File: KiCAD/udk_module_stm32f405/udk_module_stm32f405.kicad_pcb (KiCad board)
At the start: 4 copper layers, 54 x 38 mm, 33 parts, among them J1 USB_C_Receptacle, J2 5V, J3 ARGB, J4 QWIIC, J5 CONN, J6 SPI, U1 AMS1117-3.3, U2 NC7SZ125M5X, U3 STM32F405RGTx, U4 USB3300-EZK, U5 TS3USB30EDGSR

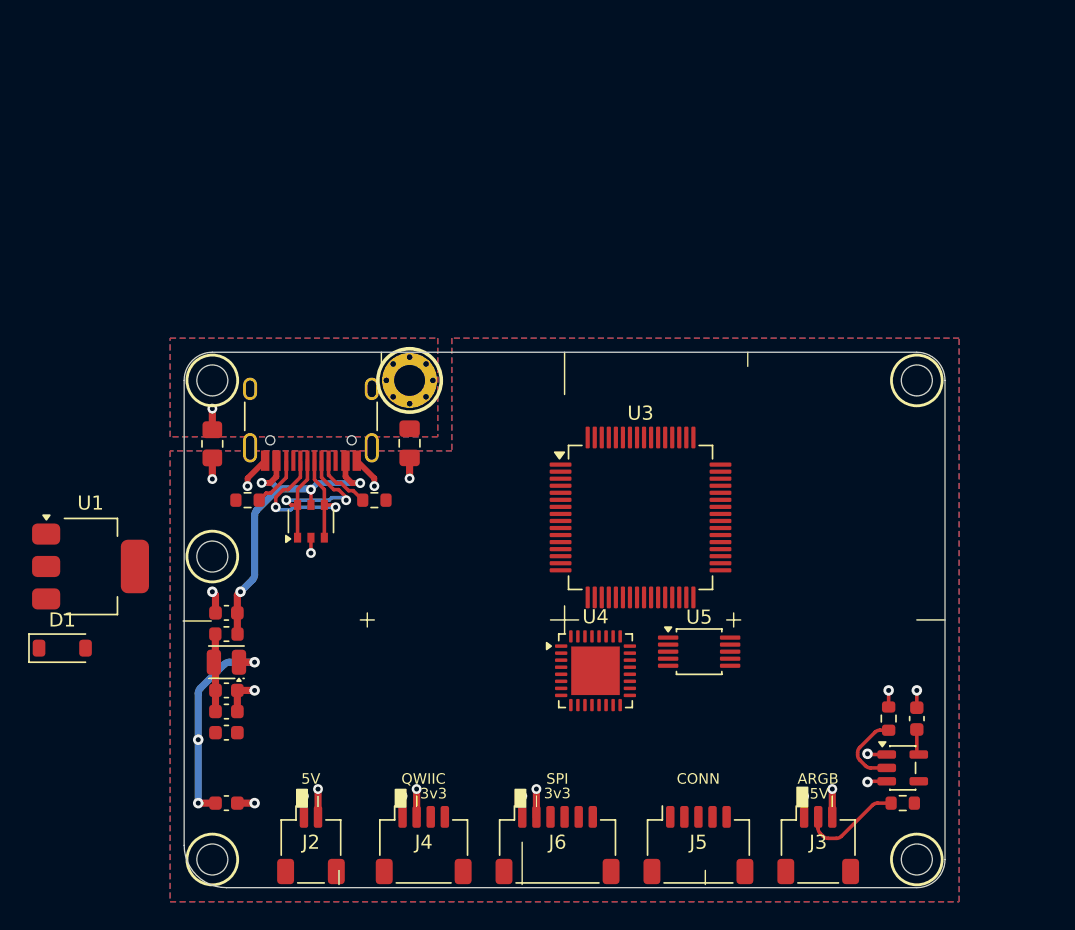
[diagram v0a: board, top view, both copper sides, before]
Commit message: wip-2025-11-27
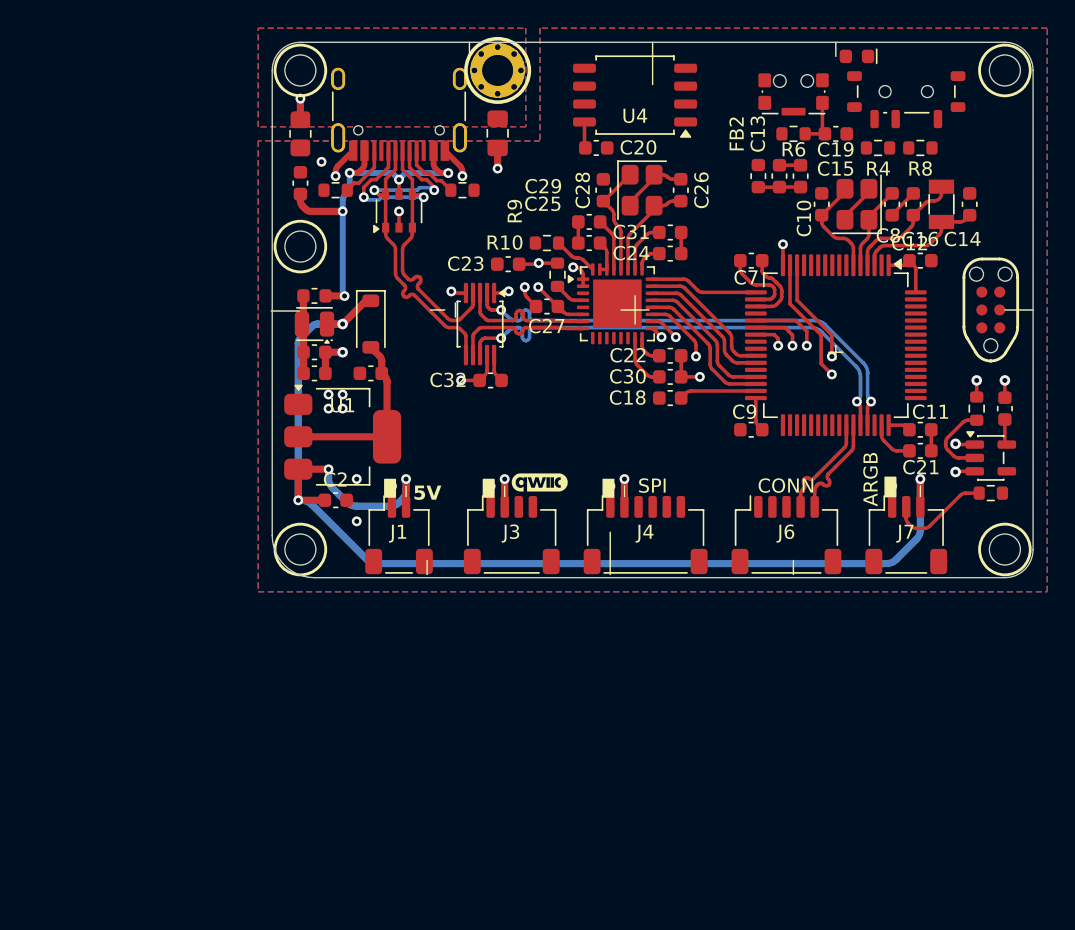
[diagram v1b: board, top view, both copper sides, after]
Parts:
- removed the U3 at (102.4, 81.7)
- added BOOT1: SW-BOOT, Button_Switch_SMD:SW_SPDT_Shouhan_MSK12C02, F.Cu at (121.2, 51.5)
- added C10: 20p, Capacitor_SMD:C_0603_1608Metric, F.Cu at (115.2, 59.5)
- added C11: 100n, Capacitor_SMD:C_0603_1608Metric, F.Cu at (122.2, 75.5)
- added C12: 100n, Capacitor_SMD:C_0603_1608Metric, F.Cu at (122.2, 63.5)
- added C13: 10n, Capacitor_SMD:C_0603_1608Metric, F.Cu at (112.2, 57.5)
- added C14: 12p, Capacitor_SMD:C_0603_1608Metric, F.Cu at (125.8, 59.5)
- added C15: 1u, Capacitor_SMD:C_0603_1608Metric, F.Cu at (113.8, 57.5)
- added C16: 12p, Capacitor_SMD:C_0603_1608Metric, F.Cu at (121.8, 59.5)
- added C18: 2u2, Capacitor_SMD:C_0603_1608Metric, F.Cu at (104.5, 73.2)
- added C19: 100n, Capacitor_SMD:C_0603_1608Metric, F.Cu at (116.2, 54.5)
- added C20: 100n, Capacitor_SMD:C_0603_1608Metric, F.Cu at (99.2, 55.5)
- added C21: 2u2, Capacitor_SMD:C_0603_1608Metric, F.Cu at (122.2, 77.0)
- added C22: 100n, Capacitor_SMD:C_0603_1608Metric, F.Cu at (104.5, 70.2)
- added C23: 1u, Capacitor_SMD:C_0603_1608Metric, F.Cu at (93.0, 63.8)
- added C24: 100n, Capacitor_SMD:C_0603_1608Metric, F.Cu at (104.5, 63.0)
- added C25: 100n, Capacitor_SMD:C_0603_1608Metric, F.Cu at (98.8, 62.2)
- added C26: 9p, Capacitor_SMD:C_0603_1608Metric, F.Cu at (105.2, 58.5)
- added C27: 100n, Capacitor_SMD:C_0603_1608Metric, F.Cu at (95.8, 66.8)
- added C28: 9p, Capacitor_SMD:C_0603_1608Metric, F.Cu at (99.8, 58.5)
- added C29: 4u7, Capacitor_SMD:C_0603_1608Metric, F.Cu at (98.8, 60.8)
- added C30: 4u7, Capacitor_SMD:C_0603_1608Metric, F.Cu at (104.5, 71.8)
- added C31: 4u7, Capacitor_SMD:C_0603_1608Metric, F.Cu at (104.5, 61.5)
- added C32: 100n, Capacitor_SMD:C_0603_1608Metric, F.Cu at (91.8, 72.0)
- added C7: 100n, Capacitor_SMD:C_0603_1608Metric, F.Cu at (110.2, 63.5)
- added C8: 20p, Capacitor_SMD:C_0603_1608Metric, F.Cu at (120.2, 59.5)
- added C9: 100n, Capacitor_SMD:C_0603_1608Metric, F.Cu at (110.2, 75.5)
- added D2: Blue, PCM_SparkFun-LED:LED_0603_1608Metric_Blue, F.Cu at (117.8, 49.0)
- added FB2: 1kΩ@100MHz, Inductor_SMD:L_0603_1608Metric, F.Cu at (110.8, 57.5)
- added G***: LOGO, PCM_SparkFun-Aesthetic:qwiic_4mm, F.Cu at (95.2, 79.2)
- added J5: TC2030_SWD, PCM_marbastlib-various:CON_TC2030_outlined, F.Cu at (127.2, 67.0)
- added R10: 12K, Resistor_SMD:R_0603_1608Metric, F.Cu at (95.8, 62.2)
- added R4: 10K, Resistor_SMD:R_0603_1608Metric, F.Cu at (119.2, 55.5)
- added R6: 10K, Resistor_SMD:R_0603_1608Metric, F.Cu at (113.2, 54.5)
- added R8: 10K, Resistor_SMD:R_0603_1608Metric, F.Cu at (122.2, 55.5)
- added R9: 820R, Resistor_SMD:R_0603_1608Metric, F.Cu at (96.5, 64.5)
- added U2: STM32F405RGTx, Package_QFP:LQFP-64_10x10mm_P0.5mm, F.Cu at (116.2, 69.5)
- added U6: USB3300-EZK, Package_DFN_QFN:QFN-32-1EP_5x5mm_P0.5mm_EP3.45x3.45mm, F.Cu at (100.8, 66.6)
- added Y1: 25MHz 20pF SMD3225-4P, Crystal:Crystal_SMD_3225-4Pin_3.2x2.5mm, F.Cu at (117.8, 59.5)
- added Y2: 32.768kHz 12.5pF SMD3215-2P, Crystal:Crystal_SMD_3215-2Pin_3.2x1.5mm, F.Cu at (123.8, 59.5)
- added Y3: 24MHz, Crystal:Crystal_SMD_3225-4Pin_3.2x2.5mm, F.Cu at (102.5, 58.5)
- added ~{RST}1: SW-RESET, Button_Switch_SMD:SW_SPST_CK_KMS2xxGP, F.Cu at (113.2, 51.5)
- C1: renamed from C4; footprint PCM_SparkFun-Capacitor:C_0603_1608Metric -> Capacitor_SMD:C_0603_1608Metric
- C17: renamed from C7; footprint PCM_SparkFun-Capacitor:C_0603_1608Metric -> Capacitor_SMD:C_0603_1608Metric
- C2: footprint PCM_SparkFun-Capacitor:C_0603_1608Metric -> Capacitor_SMD:C_0603_1608Metric
- C4: renamed from C5; footprint PCM_SparkFun-Capacitor:C_0603_1608Metric -> Capacitor_SMD:C_0603_1608Metric
- C5: renamed from C6; footprint PCM_SparkFun-Capacitor:C_0603_1608Metric -> Capacitor_SMD:C_0603_1608Metric
- C6: renamed from C3; footprint PCM_SparkFun-Capacitor:C_0603_1608Metric -> Capacitor_SMD:C_0603_1608Metric
- U4: value USB3300-EZK -> MB85RS64; footprint Package_DFN_QFN:QFN-32-1EP_5x5mm_P0.5mm_EP3.45x3.45mm -> Package_SO:SOIC-8_5.3x5.3mm_P1.27mm
- moved U4 41.0 mm to (102.0, 51.8), turned to 180 degrees
- moved D1 31.8 mm to (83.2, 68.0), turned to -90 degrees
- moved C1 30.9 mm to (78.2, 58.0), turned to 90 degrees
- moved U5 28.0 mm to (91.0, 68.0), turned to -90 degrees
- moved C6 27.5 mm to (83.2, 71.5)
- moved C4 24.8 mm to (79.2, 70.0)
- moved C5 24.8 mm to (79.2, 71.5)
- moved FB1 24.8 mm to (79.2, 66.0)
- moved PTC1 24.8 mm to (79.2, 68.0)
- moved C3 22.9 mm to (92.2, 54.5)
- moved J2 22.9 mm to (85.2, 51.6)
- moved C17 22.9 mm to (128.2, 74.0)
- moved H1 22.9 mm to (92.2, 50.0)
- moved H2 22.9 mm to (128.2, 50.0)
- moved H3 22.9 mm to (128.2, 84.0)
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- renumbered C1 to C3, J2 to J1, J1 to J2, J4 to J3, J6 to J4, J5 to J6, J3 to J7, R3 to R1, R1 to R2, R2 to R3, R4 to R5, R5 to R7, U2 to U3
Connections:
- C6 pad 1: +3.3V -> +3V3
- D1 pad 2: +3.3V -> +3V3
- J3 pad 2: +3.3V -> +3V3
- J4 pad 2: +3.3V -> +3V3
- J4 pad 4: PICO -> MISO
- J4 pad 5: POCI -> MOSI
- J4 pad 6: SS -> SS/MATRIX-CS
- J6 pad 1: CON1 -> ADC1/WKUP/CON1
- J6 pad 2: CON2 -> ADC2/CON2
- J6 pad 3: CON3 -> RGB-EN/ADC3
- R5 pad 1: unconnected-(R4-Pad1) -> RGB
- U1 pad 2: +3.3V -> +3V3
- U4 pad 1: unconnected-(U4-GND-Pad1) -> EEPROM-CS
- U4 pad 2: unconnected-(U4-GND-Pad2) -> MISO
- U4 pad 3: unconnected-(U4-CPEN-Pad3) -> GND
- U4 pad 4: unconnected-(U4-VBUS-Pad4) -> GND
- U4 pad 5: unconnected-(U4-ID-Pad5) -> MOSI
- U4 pad 6: unconnected-(U4-VDD3.3-Pad6) -> SCK
- U4 pad 7: unconnected-(U4-DP-Pad7) -> GND
- U4 pad 8: unconnected-(U4-DM-Pad8) -> +3V3
- U5 pad 1: unconnected-(U5-S-Pad1) -> USB_SELECT
- U5 pad 10: unconnected-(U5-VCC-Pad10) -> +3V3
- U5 pad 2: unconnected-(U5-D1+-Pad2) -> USB-D1+
- U5 pad 3: unconnected-(U5-D2+-Pad3) -> USB-D2+
- U5 pad 4: unconnected-(U5-D+-Pad4) -> D+
- U5 pad 5: unconnected-(U5-GND-Pad5) -> GND
- U5 pad 6: unconnected-(U5-D--Pad6) -> D-
- U5 pad 7: unconnected-(U5-D2--Pad7) -> USB-D2-
- U5 pad 8: unconnected-(U5-D1--Pad8) -> USB-D1-
- U5 pad 9: unconnected-(U5-~{OE}-Pad9) -> GND
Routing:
- net +5V: track 20.9 -> 92.6 mm, vias 5 -> 6
- net +3V3: track 0.00 -> 45.0 mm, vias 0 -> 3
- net USB-D1+: track 0.00 -> 35.0 mm, vias 0 -> 2
- net USB-D1-: track 0.00 -> 34.8 mm, vias 0 -> 2
- net GND: track 24.2 -> 51.8 mm, vias 15 -> 24
- net D-: track 14.8 -> 27.3 mm
- net D+: track 15.2 -> 27.3 mm
- net DATA3: track 0.00 -> 10.4 mm
- net DATA4: track 0.00 -> 10.4 mm
- net USB-D2-: track 0.00 -> 9.96 mm
- net USB-D2+: track 0.00 -> 9.96 mm
- net DATA1: track 0.00 -> 9.93 mm
- net DATA2: track 0.00 -> 9.93 mm
- net OSC32-IN: track 0.00 -> 9.05 mm
- net ADC2/CON2: track 0.00 -> 8.98 mm, vias 0 -> 1
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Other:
- board text added: "D1"
- board text removed: "3v3"
- board text removed: "QWIIC"
